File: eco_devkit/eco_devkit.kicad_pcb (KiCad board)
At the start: 2 copper layers, 100 x 82 mm, 92 parts, among them J10 Micro_SD_Card_Det1, J11 DISPLAY FFC, J2 Conn_02x20_Counter_Clockwise, J3 ADC_SEL1, J4 BluetoothHeader, J8 USB_C_Receptacle_USB2.0_16P, J9 SWD Interface, Q1 MOSFET, Q2 MMBT3904, Q3 MOSFET, Q4 OP598A, Q5 T2N7002AK,LM, Q6 SL2301S, SW3 PTS636, SW4 PTS636, SW5 PTS636, SW6 PTS636, U1 RP2040, U2 LTR-329ALS-01, U3 MC3419, Y2 ABM8-272-T3

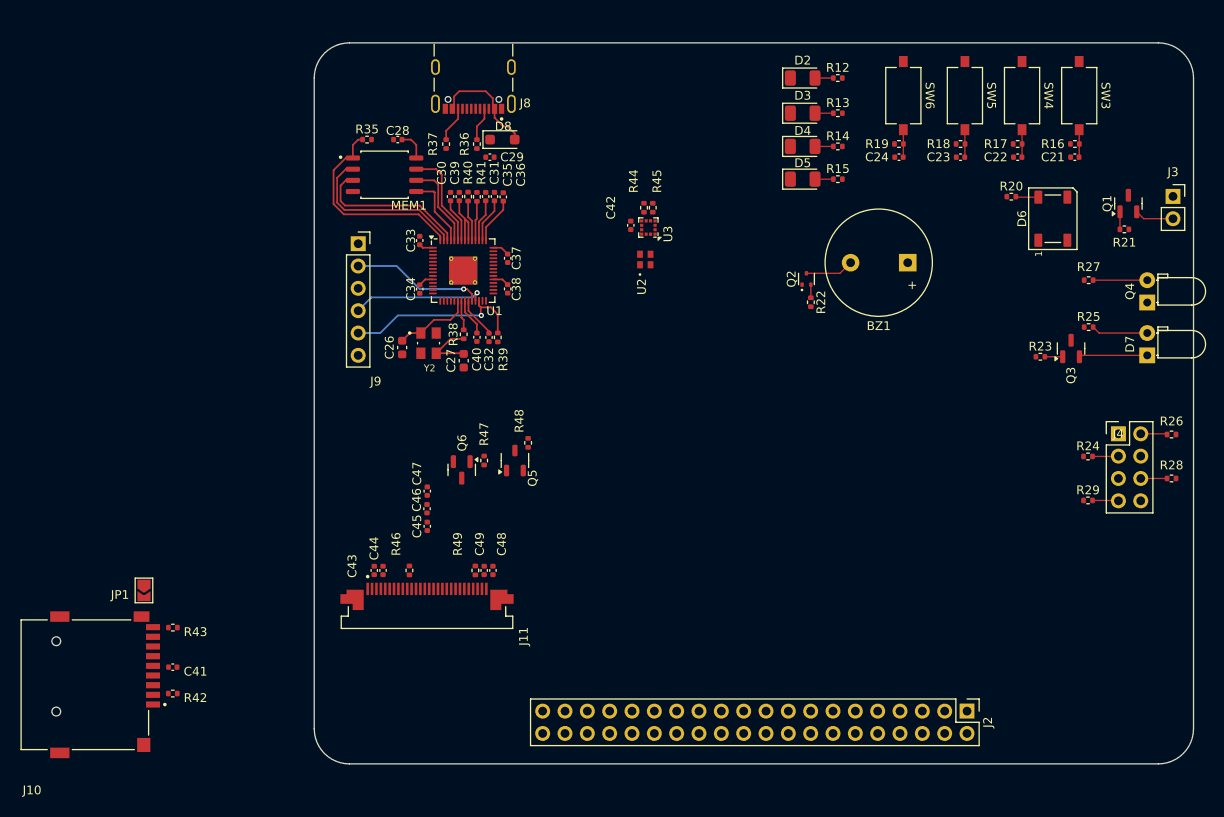
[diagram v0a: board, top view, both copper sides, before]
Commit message: Placement v1.
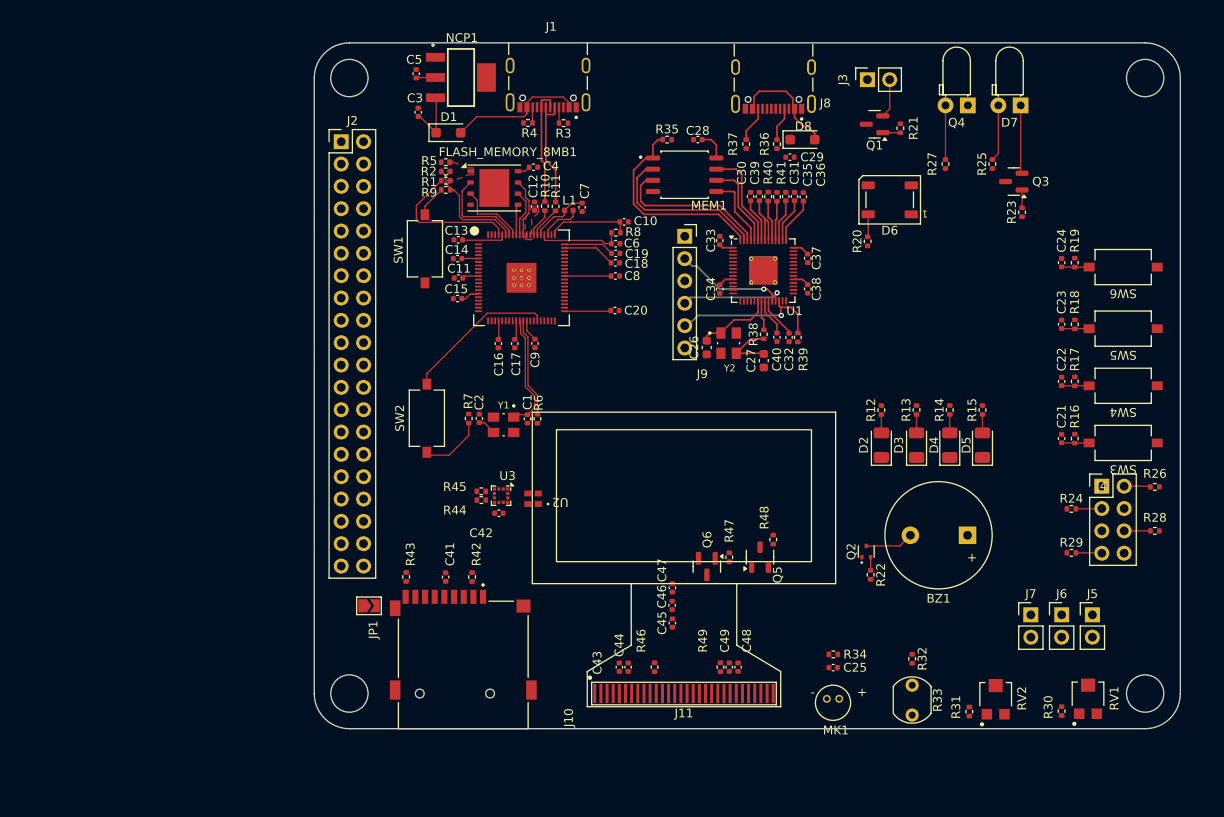
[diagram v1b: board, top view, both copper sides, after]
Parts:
- added C1: 15p, Capacitor_SMD:C_0402_1005Metric, F.Cu at (124.2, 92.8)
- added C10: 4.7u, Capacitor_SMD:C_0402_1005Metric, F.Cu at (135.2, 70.4)
- added C11: 100n, Capacitor_SMD:C_0402_1005Metric, F.Cu at (116.4, 76.8)
- added C12: 100n, Capacitor_SMD:C_0402_1005Metric, F.Cu at (125.0, 68.6)
- added C13: 100n, Capacitor_SMD:C_0402_1005Metric, F.Cu at (116.4, 72.4)
- added C14: 100n, Capacitor_SMD:C_0402_1005Metric, F.Cu at (116.3, 74.5)
- added C15: 100n, Capacitor_SMD:C_0402_1005Metric, F.Cu at (116.3, 79.1)
- added C16: 100n, Capacitor_SMD:C_0402_1005Metric, F.Cu at (120.9, 84.2)
- added C17: 100n, Capacitor_SMD:C_0402_1005Metric, F.Cu at (122.8, 84.2)
- added C18: 100n, Capacitor_SMD:C_0402_1005Metric, F.Cu at (134.2, 75.0)
- added C19: 100n, Capacitor_SMD:C_0402_1005Metric, F.Cu at (134.3, 73.9)
- added C2: 15p, Capacitor_SMD:C_0402_1005Metric, F.Cu at (118.8, 92.7)
- added C20: 100n, Capacitor_SMD:C_0402_1005Metric, F.Cu at (134.2, 80.4)
- added C25: 1u, Capacitor_SMD:C_0402_1005Metric, F.Cu at (159.0, 121.0)
- added C3: 10u, Capacitor_SMD:C_0402_1005Metric, F.Cu at (111.8, 57.9)
- added C4: 100n, Capacitor_SMD:C_0402_1005Metric, F.Cu at (124.9, 64.1)
- added C5: 10u, Capacitor_SMD:C_0402_1005Metric, F.Cu at (111.6, 53.5)
- added C6: 4.7u, Capacitor_SMD:C_0402_1005Metric, F.Cu at (134.3, 72.8)
- added C7: 4.7u, Capacitor_SMD:C_0402_1005Metric, F.Cu at (130.5, 68.7)
- added C8: 100n, Capacitor_SMD:C_0402_1005Metric, F.Cu at (134.2, 76.5)
- added C9: 4.7u, Capacitor_SMD:C_0402_1005Metric, F.Cu at (125.1, 84.2)
- added D1: SB120, Diode_SMD:D_SOD-123F, F.Cu at (115.3, 60.2)
- added FLASH_MEMORY_8MB1: W25Q80DVSSIG, Package_SON:WSON-8-1EP_6x5mm_P1.27mm_EP3.4x4.3mm, F.Cu at (120.5, 66.5)
- added J1: USB_C_Receptacle_USB2.0_16P, lib:UJ20-C-H-G-SMT-1-P16-TR, F.Cu at (126.6, 50.0)
- added J5: ADC_SEL1, Connector_PinHeader_2.54mm:PinHeader_1x02_P2.54mm_Vertical, F.Cu at (188.5, 115.0)
- added J6: ADC_SEL1, Connector_PinHeader_2.54mm:PinHeader_1x02_P2.54mm_Vertical, F.Cu at (185.0, 115.0)
- added J7: ADC_SEL1, Connector_PinHeader_2.54mm:PinHeader_1x02_P2.54mm_Vertical, F.Cu at (181.5, 115.0)
- added L1: 3.3u, Inductor_SMD:L_0402_1005Metric, F.Cu at (129.0, 69.1)
- added MK1: MIC, EcoDevkit:MIC_CMEJ-0415-42-P, F.Cu at (159.0, 125.0)
- added NCP1: NCP1117ST50T3G, lib:NCP1117ST50T3G, F.Cu at (116.7, 53.9)
- added R1: 0, Resistor_SMD:R_0402_1005Metric, F.Cu at (115.0, 65.7)
- added R10: 27, Resistor_SMD:R_0402_1005Metric, F.Cu at (126.2, 68.6)
- added R11: 27, Resistor_SMD:R_0402_1005Metric, F.Cu at (127.5, 68.6)
- added R2: 0, Resistor_SMD:R_0402_1005Metric, F.Cu at (115.0, 64.6)
- added R3: 5.1k, Resistor_SMD:R_0402_1005Metric, F.Cu at (128.3, 59.1)
- added R30: 1k, Resistor_SMD:R_0402_1005Metric, F.Cu at (185.0, 126.0)
- added R31: 1k, Resistor_SMD:R_0402_1005Metric, F.Cu at (174.5, 126.0)
- added R32: 33k, Resistor_SMD:R_0402_1005Metric, F.Cu at (168.0, 120.0)
- added R33: 500k, OptoDevice:R_LDR_5.1x4.3mm_P3.4mm_Vertical, F.Cu at (168.0, 123.0)
- added R34: 2.2k, Resistor_SMD:R_0402_1005Metric, F.Cu at (159.0, 119.5)
- added R4: 5.1k, Resistor_SMD:R_0402_1005Metric, F.Cu at (124.3, 59.1)
- added R5: 10k, Resistor_SMD:R_0402_1005Metric, F.Cu at (115.0, 63.6)
- added R6: 1k, Resistor_SMD:R_0402_1005Metric, F.Cu at (125.4, 92.8)
- added R7: 1k, Resistor_SMD:R_0402_1005Metric, F.Cu at (117.6, 92.7)
- added R8: 33, Resistor_SMD:R_0402_1005Metric, F.Cu at (134.3, 71.6)
- added R9: 1k, Resistor_SMD:R_0402_1005Metric, F.Cu at (115.0, 66.7)
- added RP2350B1: RP2350B1, lib:RP2350B_QFN-80_EP_10.573x10.573_Pitch0.4mm, F.Cu at (123.6, 76.7)
- added RV1: 100k, EcoDevkit:TRIM_TC33X-2-203E, F.Cu at (188.0, 124.5)
- added RV2: 100k, EcoDevkit:TRIM_TC33X-2-203E, F.Cu at (177.5, 124.5)
- added SW1: BOOT, Button_Switch_SMD:SW_Tactile_SPST_NO_Straight_CK_PTS636Sx25SMTRLFS, F.Cu at (112.6, 73.4)
- added SW2: RESET, Button_Switch_SMD:SW_Tactile_SPST_NO_Straight_CK_PTS636Sx25SMTRLFS, F.Cu at (112.8, 92.7)
- added Y1: Crystal_GND24, lib:ABM8-272-T3, F.Cu at (121.5, 93.4)
- J11: footprint EcoDevkit:AMPHENOL_SFV28R-2STE1HLF -> EcoDevkit:FPC_30
- moved J2 96.2 mm to (103.1, 61.2), turned to 0 degrees
- moved J10 43.1 mm to (117.0, 120.8), turned to 0 degrees
- moved D2 42.7 mm to (164.5, 95.8), turned to 90 degrees
- moved D3 39.9 mm to (168.5, 95.8), turned to 90 degrees
- moved SW3 39.8 mm to (192.0, 95.5), turned to 180 degrees
- moved R12 38.1 mm to (164.5, 91.8), turned to 90 degrees
- moved R44 38.1 mm to (119.0, 102.0), turned to 180 degrees
- moved D4 37.9 mm to (172.3, 95.8), turned to 90 degrees
- moved R45 37.7 mm to (119.0, 101.0), turned to 180 degrees
- moved J3 37.2 mm to (162.9, 54.2), turned to 90 degrees
- moved J9 37.1 mm to (142.1, 72.0)
- moved R42 36.5 mm to (118.0, 110.8), turned to -90 degrees
- moved D5 36.5 mm to (176.0, 95.8), turned to 90 degrees
- moved C42 36.0 mm to (121.0, 103.5), turned to 180 degrees
- moved SW4 34.9 mm to (192.0, 89.0), turned to 180 degrees
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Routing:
- net +3V3: track 32.5 -> 76.5 mm
- net RUN: track 0.00 -> 17.3 mm
- net +1V1: track 14.5 -> 30.8 mm
- net PROBE_GPIO4/UART_TX: track 0.00 -> 16.1 mm
- net Net-(D1-A): track 0.00 -> 15.5 mm
- net /MCU/USB_D-: track 0.00 -> 13.8 mm
- net /MCU/XIN: track 0.00 -> 13.5 mm
- net /MCU/USB_D+: track 0.00 -> 13.5 mm
- net /MCU/QSPI_SS: track 0.00 -> 12.6 mm
- net /MCU/XOUT: track 0.00 -> 11.3 mm
- net /MCU/QSPI_SD1: track 0.00 -> 10.7 mm
- net Net-(RP2350B1-VREG_AVDD): track 0.00 -> 9.75 mm
- net /MCU/QSPI_SD2: track 0.00 -> 7.97 mm
- net Net-(R7-Pad2): track 0.00 -> 7.02 mm
- net +VBUS: track 0.00 -> 6.81 mm
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- added copper zone on F.Cu, net (none)
- added copper zone on F.Cu, net +3V3
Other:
- board size 100 x 82 mm -> 98.5 x 78 mm
